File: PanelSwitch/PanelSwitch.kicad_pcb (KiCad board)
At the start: 2 copper layers, 34.3 x 41.9 mm, 16 parts, among them J1 Conn_01x02_Male, J2 Conn_01x02_Male, J3 Conn_01x02_Male

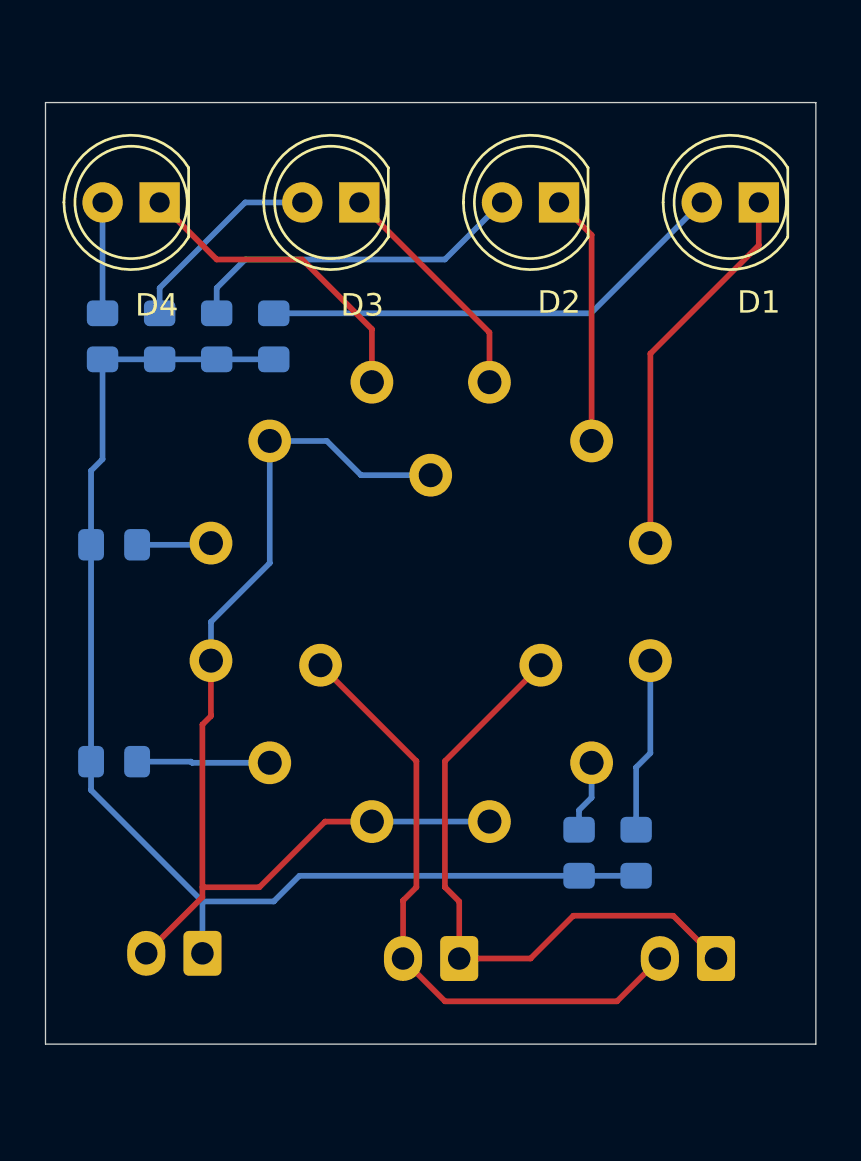
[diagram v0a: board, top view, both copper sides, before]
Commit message: Boards sent to be built.
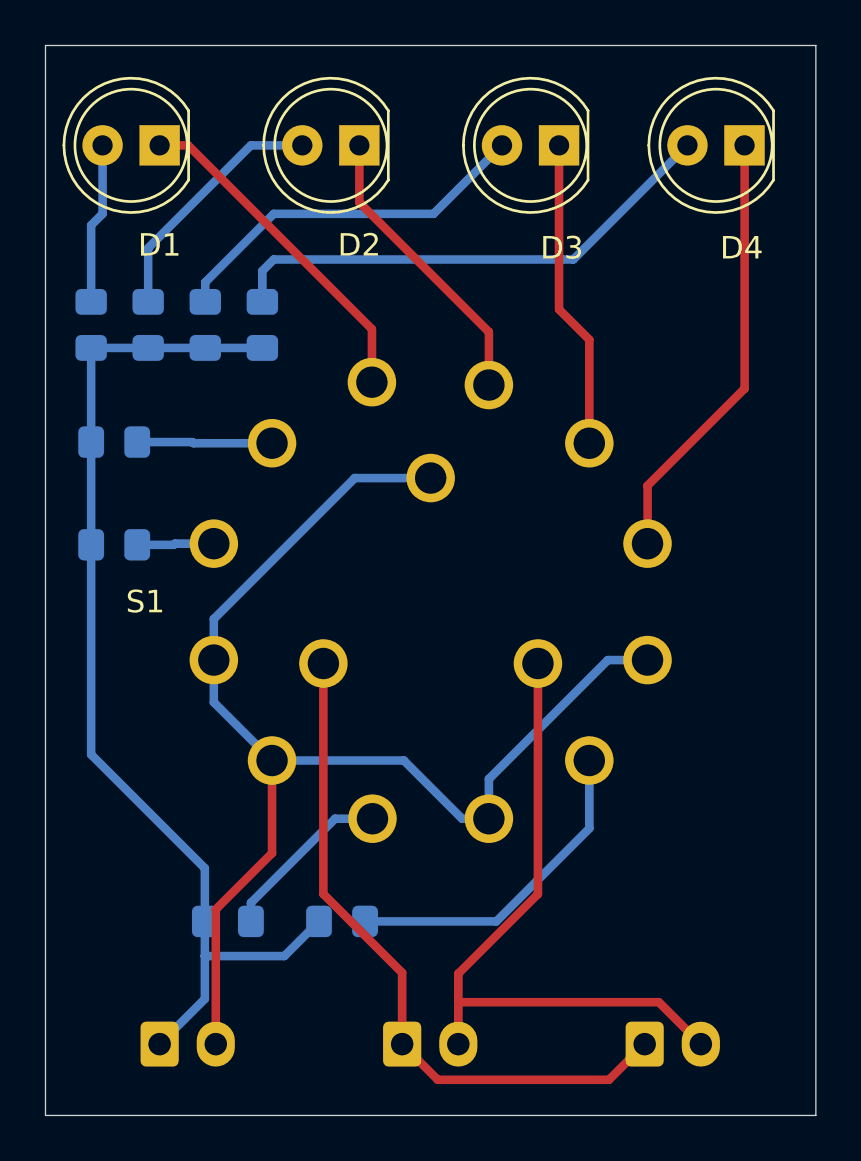
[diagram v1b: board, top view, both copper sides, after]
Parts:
- S1: moved to F.Cu
- moved R2 29.6 mm to (119.6, 85.2), turned to 0 degrees
- moved D1 26.8 mm to (121.7, 72.0)
- moved D4 26.2 mm to (147.7, 72.0)
- moved R1 24.8 mm to (119.6, 89.8), turned to 0 degrees
- moved R3 19.6 mm to (129.8, 106.5)
- moved D2 9.25 mm to (130.5, 72.0)
- moved D3 9.25 mm to (139.4, 72.0)
- moved R4 8.73 mm to (124.7, 106.5)
- moved R5 8.14 mm to (118.6, 80.0)
- moved R8 7.13 mm to (126.2, 80.0)
- moved J3 4.96 mm to (143.2, 112.0), turned to 0 degrees
- moved J2 4.58 mm to (132.4, 112.0), turned to 0 degrees
- moved J1 4.47 mm to (121.7, 112.0), turned to 0 degrees
- moved R6 3.09 mm to (121.1, 80.0)
- moved R7 2.09 mm to (123.7, 80.0)
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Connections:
- net Net-(R1-Pad2) renamed /B2
- net Net-(R2-Pad2) renamed /B3
- net Net-(R3-Pad2) renamed /A1
- net Net-(R4-Pad2) renamed /A3
- J2 pad 1: /A -> /B
- J2 pad 2: /B -> /A
- J3 pad 1: /A -> /B
- J3 pad 2: /B -> /A
- S1 pad 11: /A -> /B
- S1 pad 6: /B -> /A
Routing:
- net Net-(D4-Pad2): track 4.94 -> 22.6 mm
- net Net-(D1-Pad2): track 21.1 -> 7.18 mm
- net /A1: track 3.32 -> 14.7 mm
- net +5V: track 56.1 -> 47.3 mm
- net GND: track 46.9 -> 55.0 mm
- net Net-(D3-Pad2): track 9.05 -> 16.6 mm
- net /Led3: track 14.1 -> 19.5 mm
- net Net-(D2-Pad2): track 15.4 -> 11.1 mm
- net /Led2: track 10.4 -> 13.8 mm
- net /B: track 28.1 -> 30.5 mm
- net /Led0: track 17.2 -> 15.2 mm
- net /A: track 28.1 -> 30.0 mm
- net /A3: track 5.92 -> 7.79 mm
- net /Led1: track 11.2 -> 13.1 mm
- net /B3: track 7.79 -> 6.02 mm
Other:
- board size 34.3 x 41.9 mm -> 34.3 x 47.6 mm
- net class Default: trace_width 0.254 -> 0.381
- board text added: "0"
- board text added: "1"
- board text added: "2"
- board text added: "3"
- board text added: "A"
- board text added: "A0"
- board text added: "A1"
- board text added: "A2"
- board text added: "A3"
- board text added: "B"
- board text added: "B0"
- board text added: "B1"
- board text added: "B2"
- board text added: "B3"
